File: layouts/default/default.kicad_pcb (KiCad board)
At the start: 2 copper layers, 77 parts

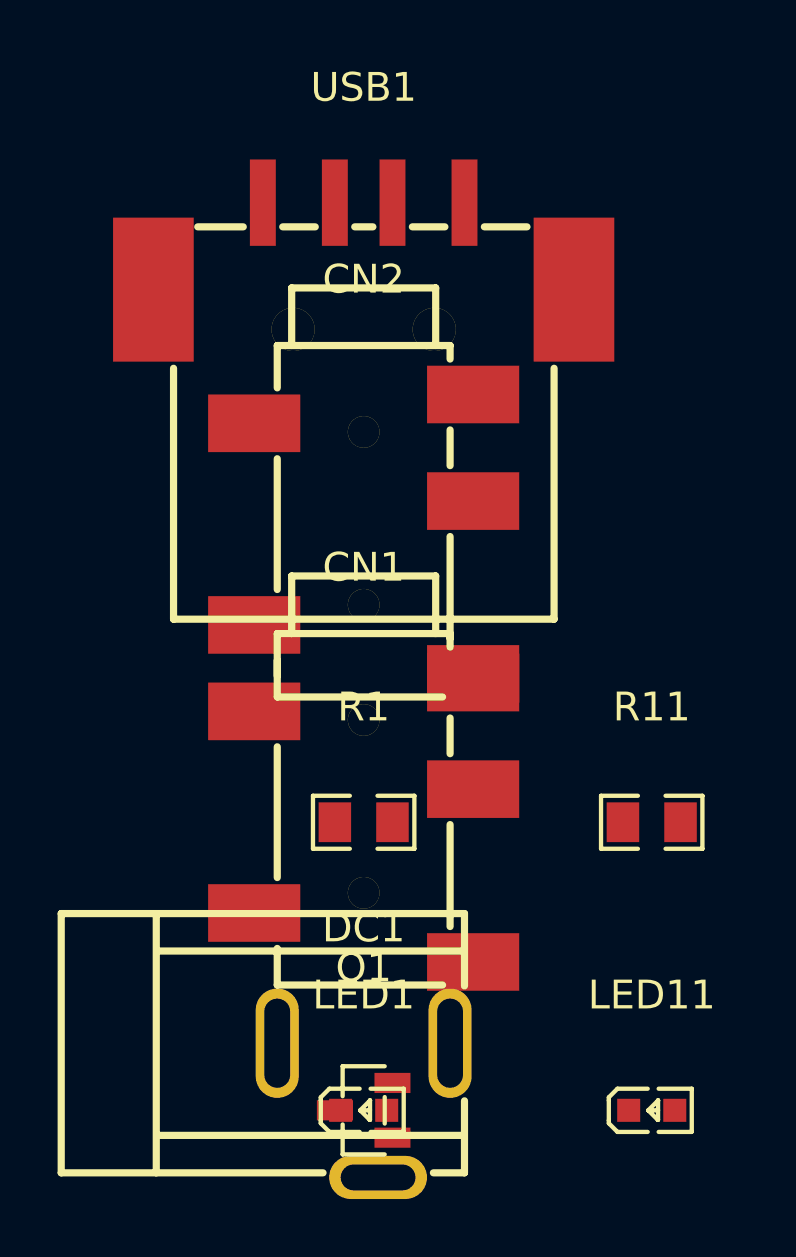
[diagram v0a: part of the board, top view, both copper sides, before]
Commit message: documentation
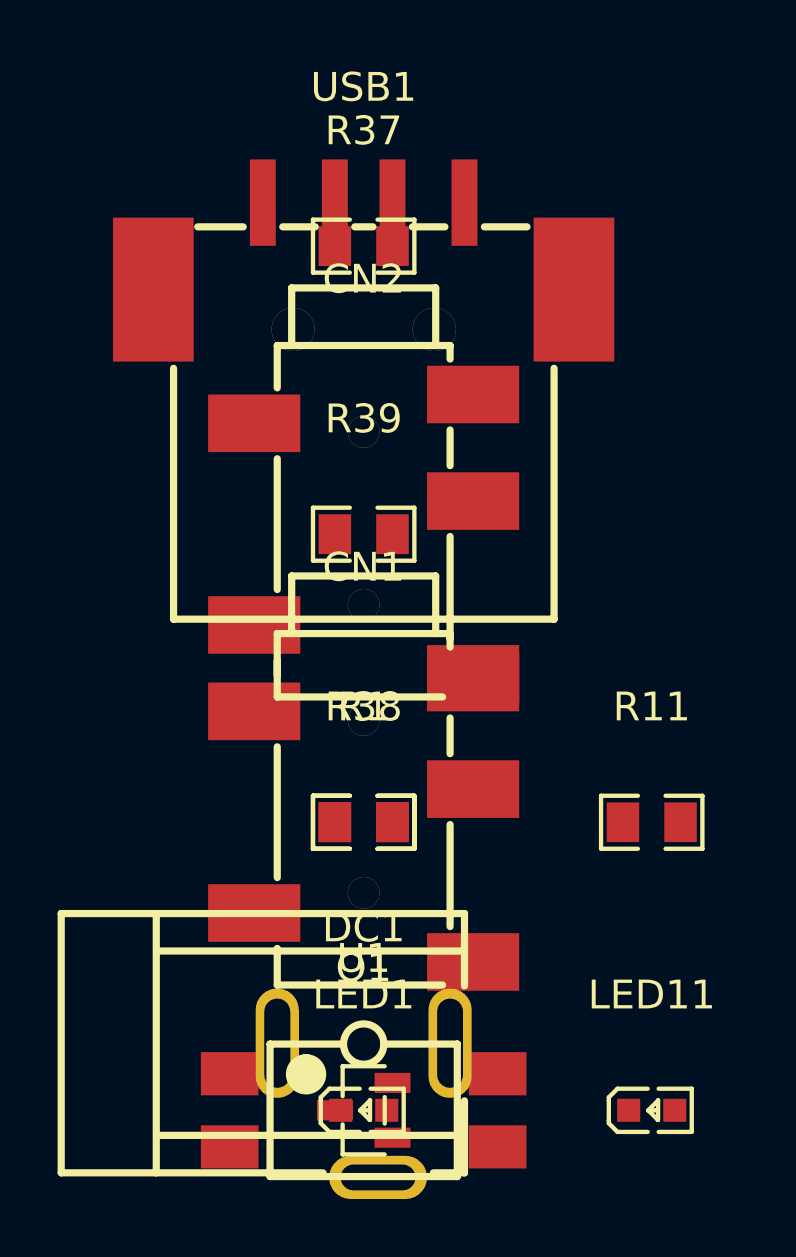
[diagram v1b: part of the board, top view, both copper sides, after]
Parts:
- added R37: , YAGEO_RC0805FR_071KL:R0805, F.Cu at (0.00, -30.0)
- added R38: , YAGEO_RC0805FR_07100RL:R0805, F.Cu at (0.00, -10.0)
- added R39: , FOJAN_FRC0805F1003TS:R0805, F.Cu at (0.00, -20.0)
- added U1: , Sharp_Microelectronics_PC817X2CSP9F:SMD-4_L4.6-W6.5-P2.54-LS10.2-TL, F.Cu at (0.00, 0.00)
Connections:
- CN1 pad 4: footprint-R-0 -> footprint-R-1
- CN2 pad 4: footprint-R-1 -> footprint-R-0

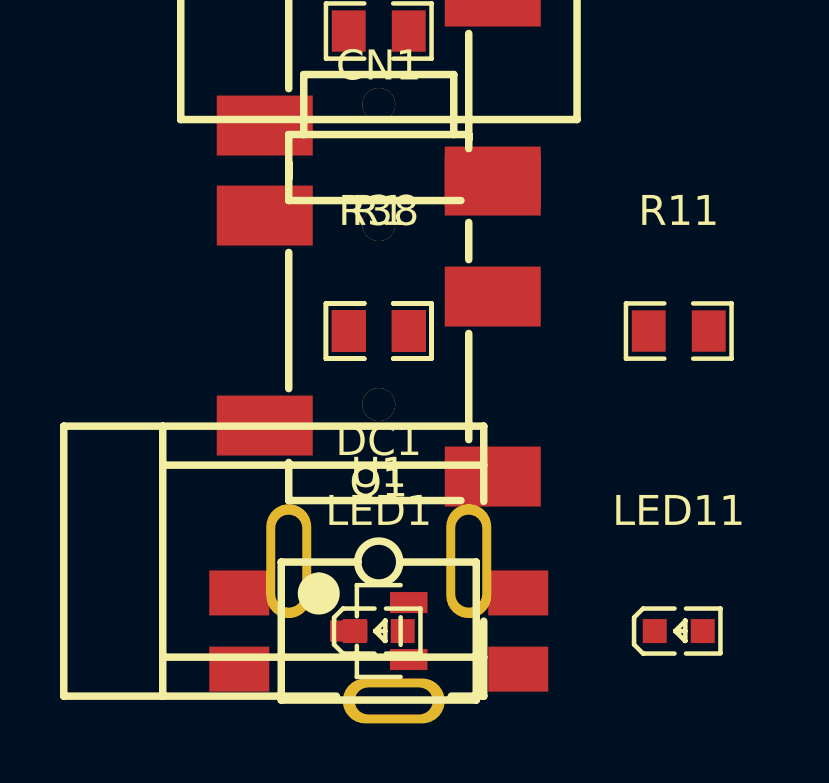
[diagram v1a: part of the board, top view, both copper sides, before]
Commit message: dont even know whats up w the max current thing
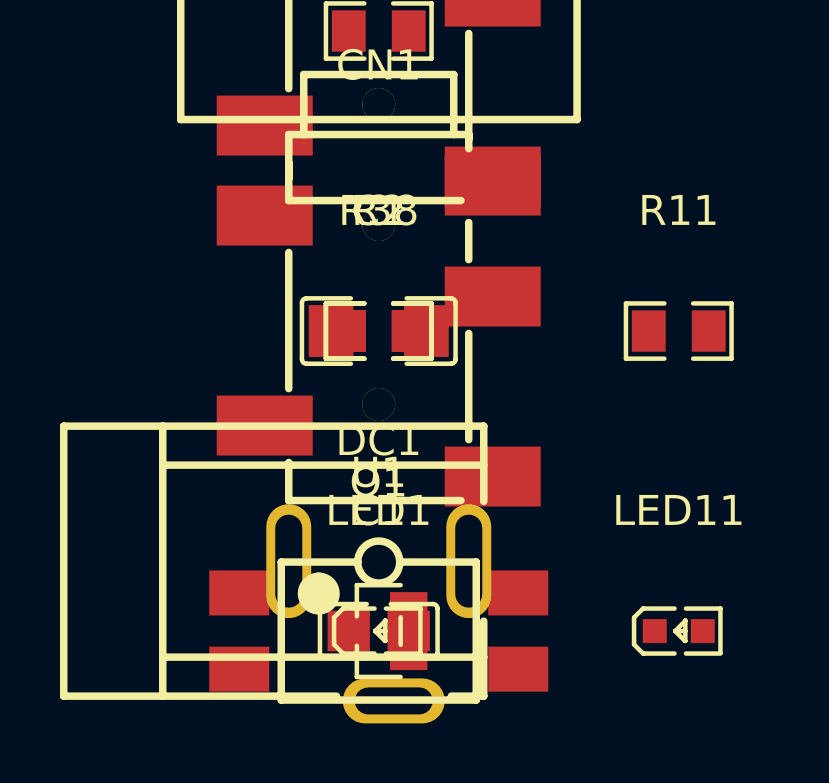
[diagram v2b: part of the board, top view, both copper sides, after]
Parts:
- added C1: , YAGEO_CC0805KRX7R9BB104:C0805, F.Cu at (0.00, 0.00)
- added C2: , Samsung_Electro_Mechanics_CL31A107MQHNNNE:C1206, F.Cu at (0.00, -10.0)
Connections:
- net footprint-R-0 renamed R
- CN1 pad 4: footprint-R-1 -> GND
